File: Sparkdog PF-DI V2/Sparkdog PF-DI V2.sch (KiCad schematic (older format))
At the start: 12 parts, among them J1 Conn_01x06_Female, J2 Conn_01x08_Female, J3 Conn_01x06_Female, J4 Conn_01x08_Female, J5 Conn_01x06_Female, U2 Arduino_Footprint

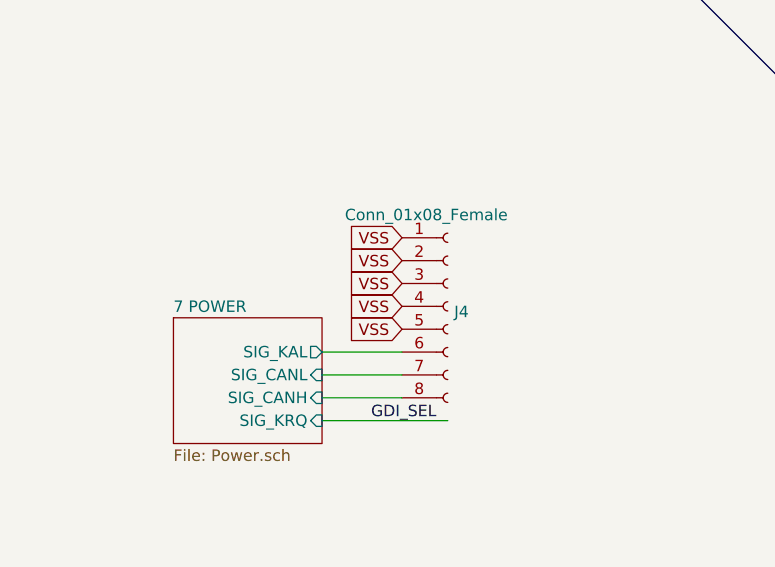
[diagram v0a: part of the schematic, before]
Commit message: Commit running changes for safekeeping
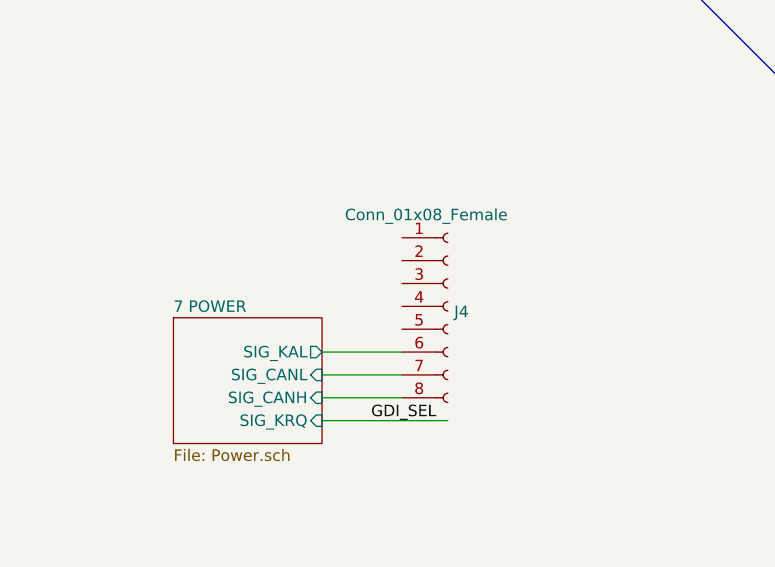
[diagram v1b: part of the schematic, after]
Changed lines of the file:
@@
 Wire Wire Line
 	3100 6600 3450 6600
-Text GLabel 3450 6100 0    50   Input ~ 0
-VSS
-Text GLabel 3450 6200 0    50   Input ~ 0
-VSS
-Text GLabel 3450 6300 0    50   Input ~ 0
-VSS
-Text GLabel 3450 6400 0    50   Input ~ 0
-VSS
-Text GLabel 3450 6500 0    50   Input ~ 0
-VSS
 Wire Wire Line
 	9950 4150 10250 4150

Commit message: Commit for safekeeping
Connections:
- wire segments 284 -> 287
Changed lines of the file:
@@
 Text Notes 12650 9900 0    157  ~ 31
 SHEET 1 MASTER\nSHEET 2 VVT\nSHEET 3 TEENSY\nSHEET 4 KNOCK\nSHEET 5 ETC\nSHEET 6 ETC PROCESSOR\nSHEET 7 POWER\nSHEET 8 GDI\nSHEET 9 GDI CONTROL
+Text GLabel 6100 5700 0    50   Input ~ 0
+VSS
+Wire Wire Line
+	6100 5550 6100 5700
+Wire Wire Line
+	6200 5700 6200 5550
+Wire Wire Line
+	6200 5700 6100 5700
 Wire Bus Line
 	11050 8150 11050 10350
